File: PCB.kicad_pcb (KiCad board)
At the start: 4 copper layers, 130.2 x 64.3 mm, 31 parts, among them J1 Conn_ARM_SWD_TagConnect_TC2030, U2 STM32L476RGTx, U3 NT3H2X11, U4 SSD1306

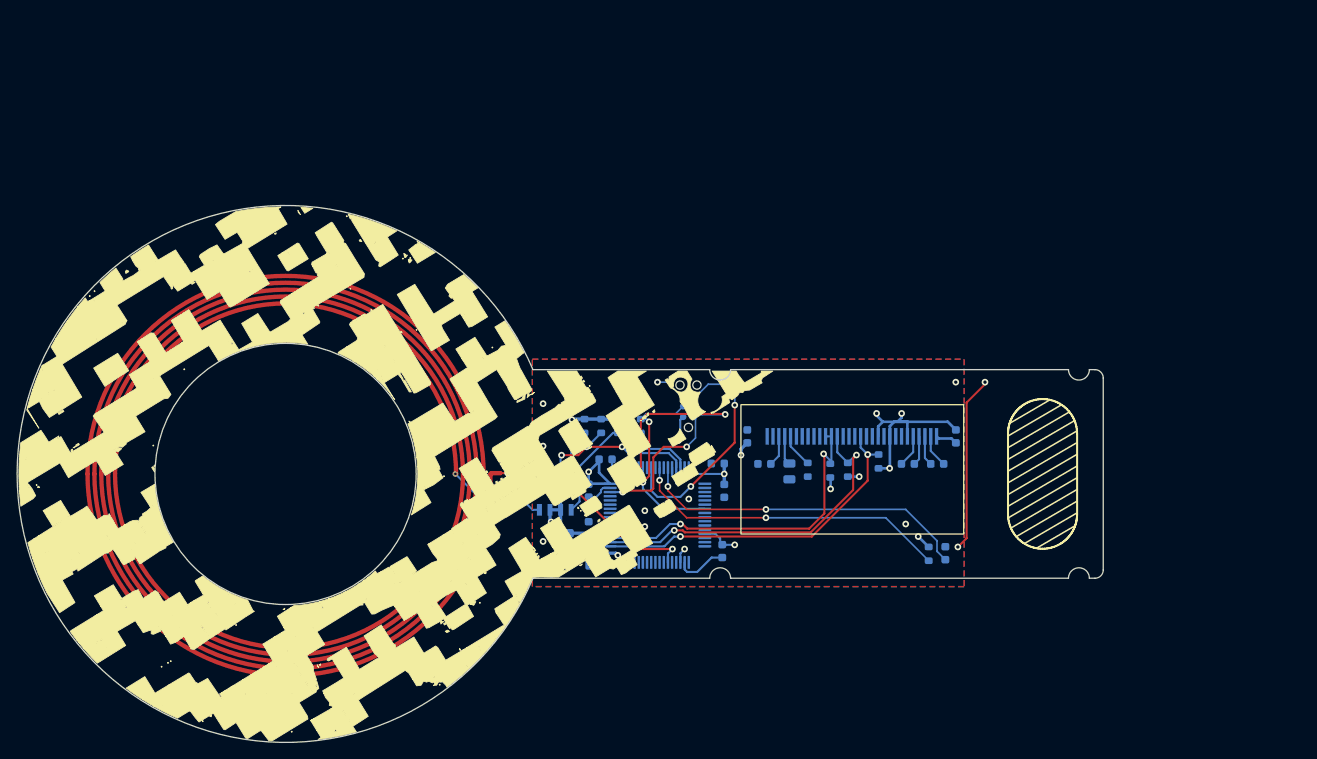
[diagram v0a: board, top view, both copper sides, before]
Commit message: TheThing PCB
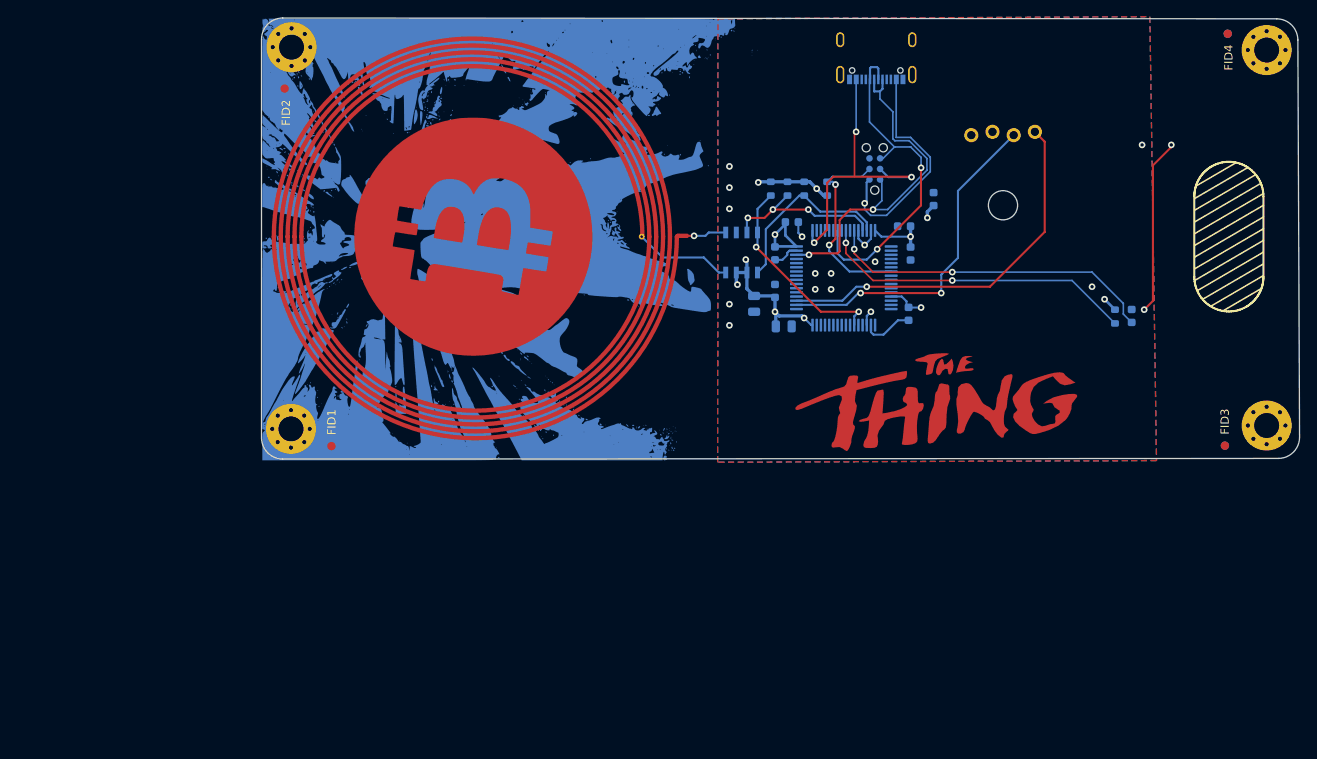
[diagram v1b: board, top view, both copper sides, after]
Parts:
- removed C10, C12, C13: 1u, Capacitor_SMD:C_0603_1608Metric
- removed C11: 4.7u, Capacitor_SMD:C_0805_2012Metric
- removed C18: ??, Capacitor_SMD:C_0603_1608Metric
- removed C7: 2.2u, Capacitor_SMD:C_0603_1608Metric
- removed R4, R6, R7: 10k, Resistor_SMD:R_0603_1608Metric
- removed R5: 390k, Resistor_SMD:R_0603_1608Metric
- removed U4: SSD1306, Footprints:OLED-128O064D-WITH-FP
- added FID1: Fiducial, Fiducial:Fiducial_1mm_Mask2mm, F.Cu at (88.2, 121.2)
- added FID2: Fiducial, Fiducial:Fiducial_1mm_Mask2mm, F.Cu at (82.6, 78.3)
- added FID3: Fiducial, Fiducial:Fiducial_1mm_Mask2mm, F.Cu at (195.3, 121.1)
- added FID4: Fiducial, Fiducial:Fiducial_1mm_Mask2mm, F.Cu at (195.6, 71.7)
- added FID5: Fiducial, Fiducial:Fiducial_1mm_Mask2mm, B.Cu at (82.6, 78.3)
- added FID6: Fiducial, Fiducial:Fiducial_1mm_Mask2mm, B.Cu at (88.2, 121.2)
- added FID7: Fiducial, Fiducial:Fiducial_1mm_Mask2mm, B.Cu at (195.6, 71.7)
- added FID8: Fiducial, Fiducial:Fiducial_1mm_Mask2mm, B.Cu at (195.3, 121.1)
- added G*** (x2): LOGO, Footprints:TheThing, F.Cu at (161.7, 116.5)
- added G*** (x2): LOGO, Footprints:btc logo, F.Cu at (105.0, 96.1)
- added G*** (x2): LOGO, Footprints:back, B.Cu at (111.2, 96.4)
- added H10: MountingHole_Pad, MountingHole:MountingHole_3mm_Pad_Via, F.Cu at (200.3, 118.7)
- added H7: MountingHole_Pad, MountingHole:MountingHole_3mm_Pad_Via, F.Cu at (83.4, 73.3)
- added H8: MountingHole, MountingHole:MountingHole_3.5mm, F.Cu at (168.7, 92.3)
- added H8: MountingHole_Pad, MountingHole:MountingHole_3mm_Pad_Via, F.Cu at (83.3, 119.1)
- added H9: MountingHole_Pad, MountingHole:MountingHole_3mm_Pad_Via, F.Cu at (200.3, 73.7)
- added J3: Conn_01x04, bitaxe:PinHeader_1x04_P2.54mm_Vertical_shifted, B.Cu at (164.9, 83.7)
- added J8: USB_C_Receptacle_USB2.0, Connector_USB:USB_C_Receptacle_GCT_USB4105-xx-A_16P_TopMnt_Horizontal, B.Cu at (153.5, 73.5)
- moved C4 36.2 mm to (157.3, 105.3)
- moved C17 36.2 mm to (160.3, 91.6)
- moved C5 36.2 mm to (156.8, 94.8)
- moved C6 36.2 mm to (157.6, 98.1)
- moved C9 36.2 mm to (138.8, 104.1)
- moved J1 36.2 mm to (153.3, 87.9)
- moved U2 36.2 mm to (149.6, 101.0)
- moved U3 36.2 mm to (137.3, 98.0)
- moved A1 36.2 mm to (105.0, 96.1)
- moved C1 36.2 mm to (142.4, 106.8)
- moved A2 36.2 mm to (194.6, 96.1)
- moved C14 36.2 mm to (184.1, 105.6)
- moved C2 36.2 mm to (143.4, 94.3)
- moved C3 36.2 mm to (141.3, 102.6)
- moved C8 36.2 mm to (141.3, 98.1)
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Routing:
- net DISP_RES: track 41.1 -> 0.00 mm, vias 2 -> 0
- net SWDIO: track 17.7 -> 42.6 mm
- net SWO: track 27.5 -> 40.7 mm
- net SWCLK: track 24.0 -> 35.6 mm, vias 2 -> 3
- net GND: track 46.4 -> 40.0 mm, vias 17 -> 16
- net DISP_SDA: track 40.1 -> 45.7 mm, vias 2 -> 1
- net Net-(U4-IREF): track 4.07 -> 0.00 mm
- net Net-(U4-C2P): track 3.94 -> 0.00 mm
- net Net-(U4-C1N): track 3.89 -> 0.00 mm
- net Net-(U4-VCC): track 3.70 -> 0.00 mm
- net Net-(U4-C2N): track 3.59 -> 0.00 mm
- net Net-(U4-C1P): track 3.53 -> 0.00 mm
- net Net-(U4-VCOMH): track 3.48 -> 0.00 mm
- net VCC: track 82.3 -> 80.1 mm, vias 17 -> 12
- net DISP_SCL: track 41.4 -> 40.5 mm
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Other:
- board size 130.2 x 64.3 mm -> 124.4 x 52.9 mm
- board text removed: "Board Rev 2C 01/25/2024"
- board text removed: "TwentyTwo Portal EA"
